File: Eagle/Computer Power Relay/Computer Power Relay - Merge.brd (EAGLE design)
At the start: 133.4 x 78 mm, 141 parts, among them K1 RELAY-3V3DC-110VAC012, K2 RELAY-110VACV3_IN-PLACE, U1 RP2040, U2 AP2112M-3.3TRG1, U3 SWITCH-SLIDE-DPDT, U4 SWITCH-SLIDE-DPDT, U5 SWITCH-SLIDE-DPDT, U6 RP2040, U7 AP2112M-3.3TRG1

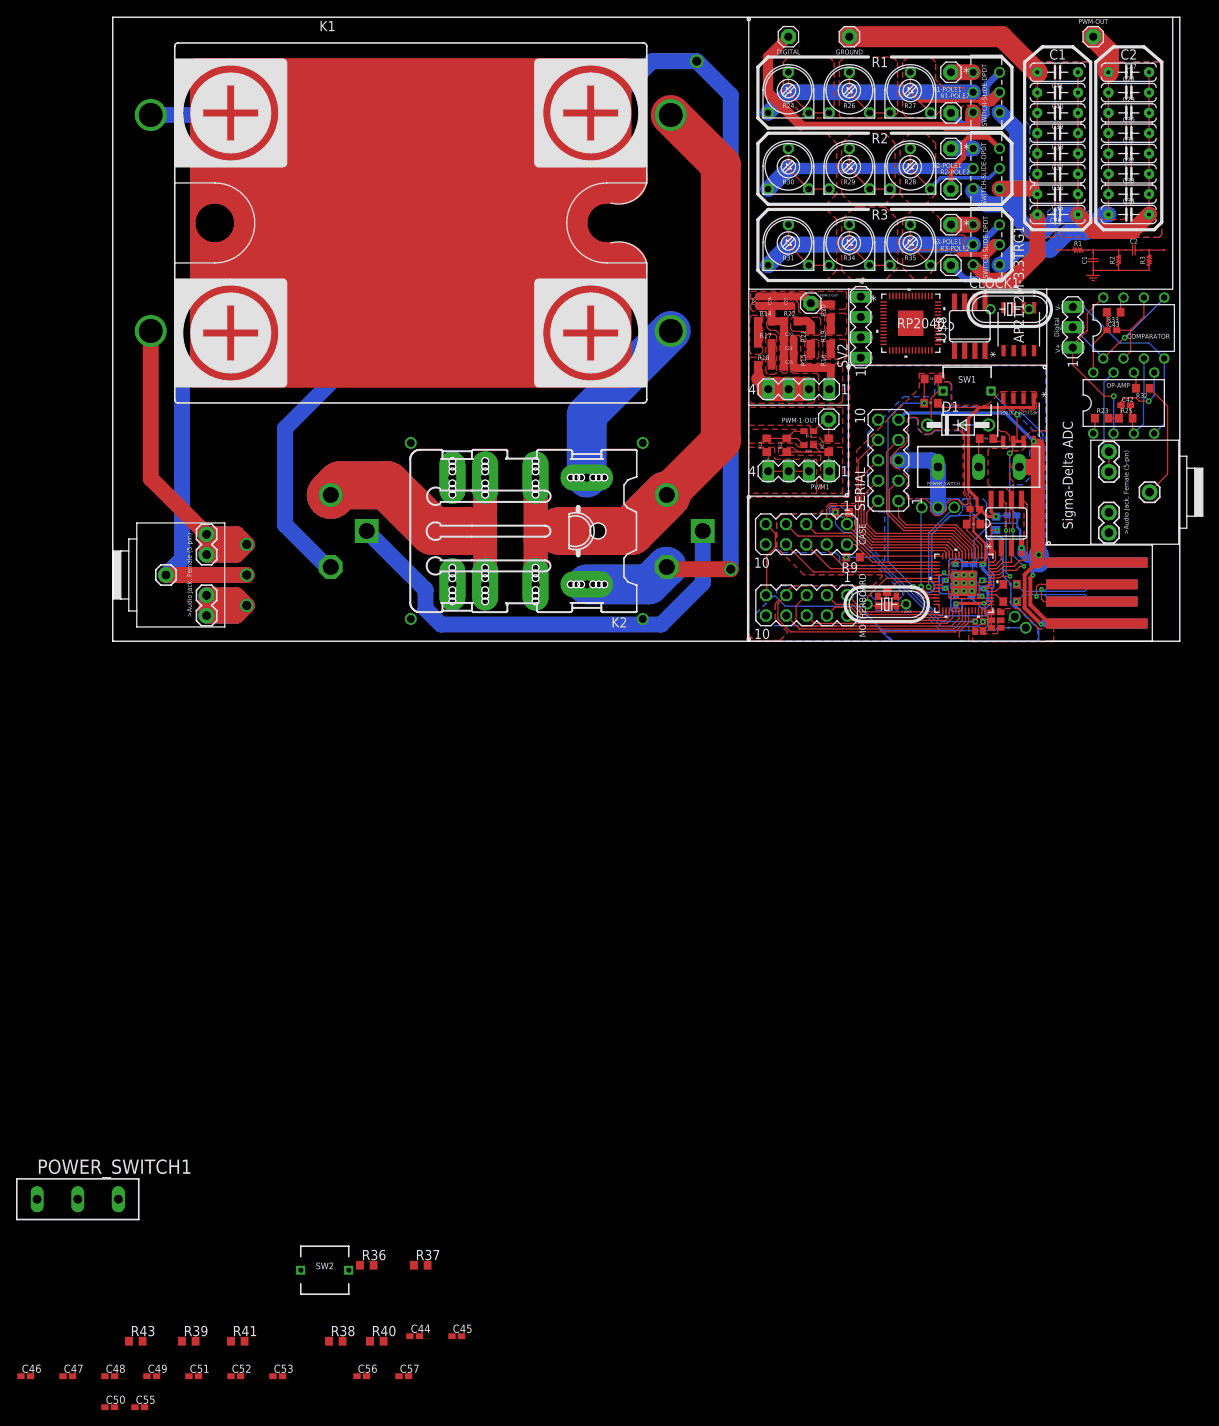
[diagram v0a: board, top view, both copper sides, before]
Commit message: CPR 100% Complete
Damn shipping's expensive.  Better work on the other projects so I can subsidize this.
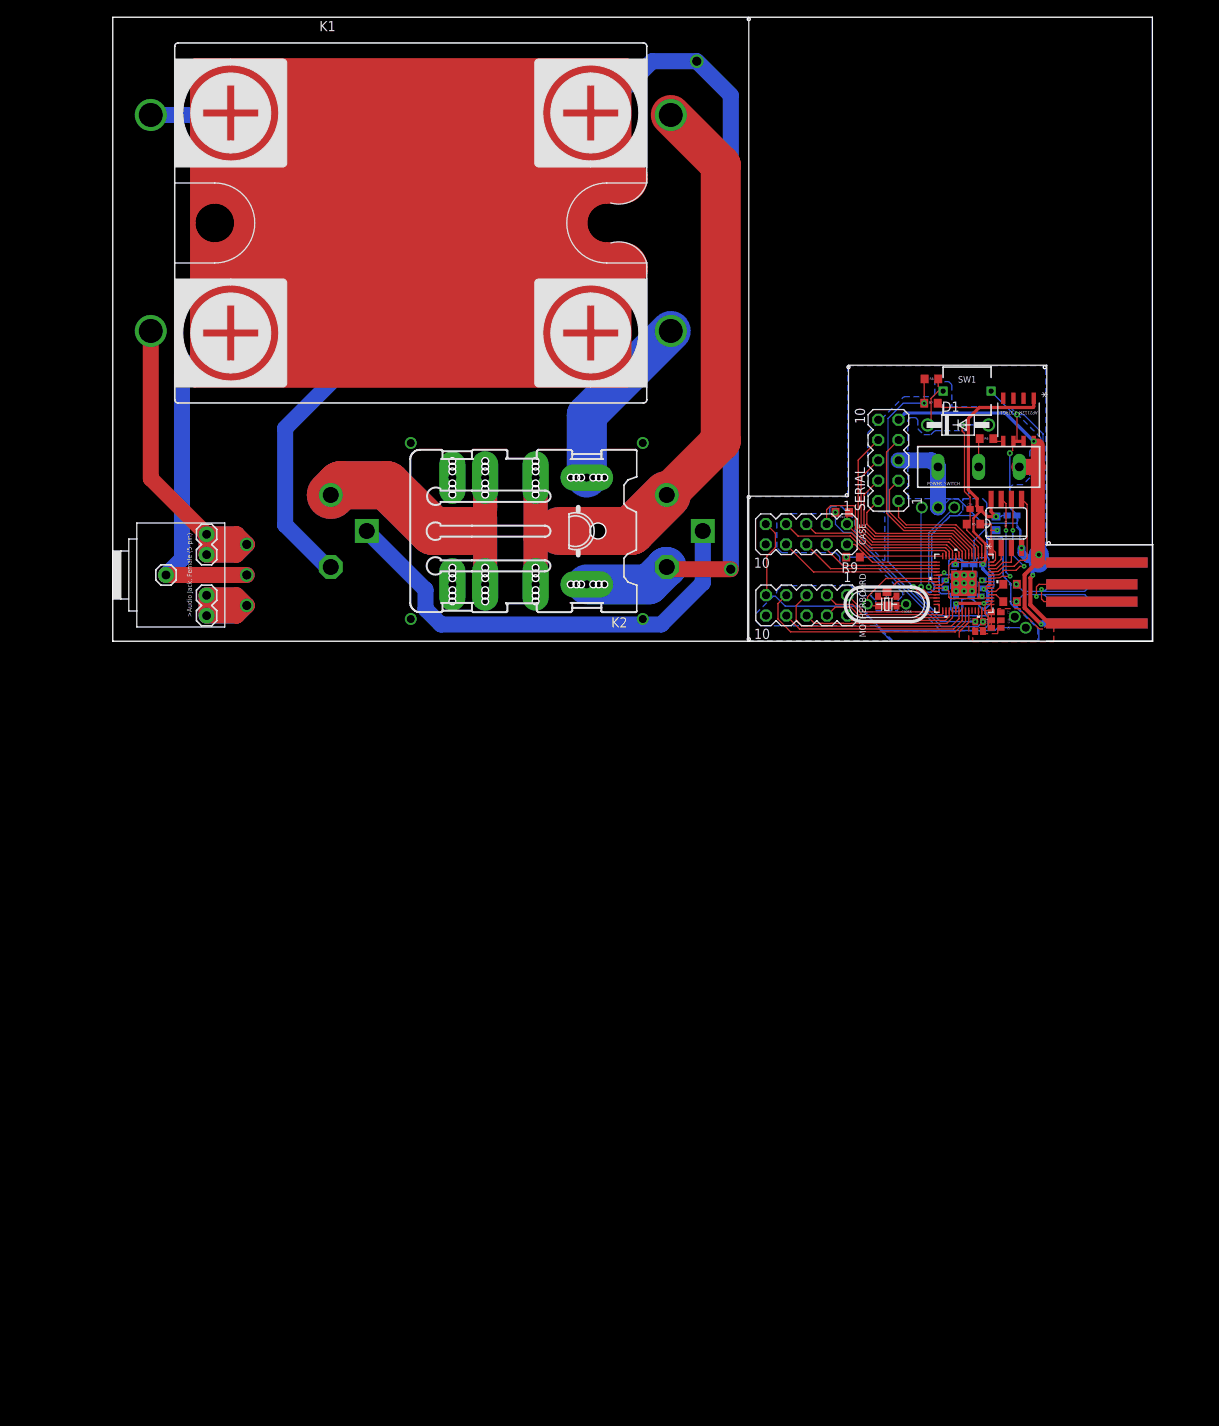
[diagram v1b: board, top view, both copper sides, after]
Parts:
- removed C18, C20, C22, C23, C46, C47, C48, C49, C51, C52, C53, C56, C57: 100nF, adafruit:C0402K
- removed C19, C21, C24, C25: 47uF, adafruit:C0402K
- removed C26, C27, C28, C29, C30, C31, C32, C33, C34, C35, C36, C37, C38, C39, C40, C41: (no value), Inventory:CAPACITOR-CERAMIC
- removed C42, C43: (no value), adafruit:C0402K
- removed C44, C45: ~30pF, adafruit:C0402K
- removed C50, C55: 1uF, adafruit:C0402K
- removed CLOCK1: 12MHz, crystal:HC49/S
- removed COMPARATOR: COMPARATOR_LM393N, Inventory:IC_2*4(8-PIN)
- removed DIGITAL, GROUND, PWM-1-OUT, PWM-2-OUT, PWM-OUT, R1-POLE1, R1-POLE2, R2-POLE1, R2-POLE2, R3-POLE1, R3-POLE2: (no value), adafruit:1X01
- removed OP-AMP: OP-AMP_TDA2822N, Inventory:IC_2*4(8-PIN)
- removed POWER_SWITCH1: SWITCH-SLIDE-2P2T, Inventory:SWITCH-SLIDE-2P2T
- removed PWM1, PWM2, SV2: (no value), con-lstb:MA04-1
- removed R11, R14, R17, R18: 220 Ω, rcl:R0603
- removed R12, R15, R21, R22: 100 Ω, rcl:R0603
- removed R13, R16, R19, R20: 1.8K Ω, rcl:R0603
- removed R23, R25, R32, R33: (no value), rcl:R0603
- removed R24, R30, R31: 1MΩ, Inventory:POTENTIOMETER_NORMAL
- removed R26, R29, R34: 10KΩ, Inventory:POTENTIOMETER_NORMAL
- removed R27, R28, R35: 100Ω, Inventory:POTENTIOMETER_NORMAL
- removed R36, R37: 27.4 Ω, rcl:R0603
- removed R38, R40: 1k Ω, rcl:R0603
- removed R39, R41: 10k Ω, rcl:R0603
- removed R43: 4.7k Ω, rcl:R0603
- removed SV1: (no value), con-lstb:MA03-1
- removed SW2: (no value), KVM Keyboard:PUSHBUTTON_TH
- removed U$6: AUDIO_JACK_FEMALE_5-PIN, Inventory:AUDIO_JACK_FEMALE_5-PIN
- removed U$8: W25Q128JVSIM-ND__QSPI-FLASH, KVM Keyboard:SO08
- removed U3, U4, U5: SWITCH-SLIDE-DPDT, Inventory:SWITCH-SLIDE-DPDT
- removed U6: RP2040, KVM Keyboard:IC57_RP2040
- removed U7: AP2112M-3.3TRG1, KVM Keyboard:AP2112M-3.3TRG1_DIO
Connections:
- removed net 5V_2: POWER_SWITCH1.1, SV2.1, U7.8
- removed net D+_2: R36.2, SV2.3
- removed net D-_2: R37.2, SV2.2
- removed net DIGITAL: COMPARATOR.1, COMPARATOR.5, SV1.2
- removed net GND-3: C18.2, PWM1.1, R12.2, R13.2
- removed net GND-4: C20.2, C22.2, C23.2, PWM2.1, R15.2, R16.2
- removed net GND-5: C26.2, C35.2, C36.2, C37.2, C38.2, C39.2, C40.2, C41.2, GROUND.1, U4.4, U5.3
- removed net GND-6: C43.2, COMPARATOR.2, COMPARATOR.6, R32.1, U$6.3
- removed net GND-7: POWER_SWITCH1.3, SV2.4, U7.6, U7.7
- removed net N$10: C19.1, PWM-1-OUT.1, R13.1
- removed net N$11: C20.1, C21.2, C22.1, C23.1, C24.2, C25.2, R14.1, R22.1
- removed net N$12: C21.1, C24.1, C25.1, PWM-2-OUT.1, R20.1
- removed net N$13: R17.1, R18.1
- removed net N$14: R14.2, R17.2
- removed net N$15: R19.2, R20.2
- removed net N$21: R16.1, R19.1
- removed net N$22: R15.1, R21.1
- removed net N$23: R21.2, R22.2
- removed net N$24: DIGITAL.1, U3.3
- removed net N$25: R24.2, R24.3, R26.1
- removed net N$26: C27.1, C28.1, C29.1, C30.1, C31.1, C32.1, C33.1, C34.1, PWM-OUT.1, U5.4
- removed net N$27: R26.2, R26.3, R27.1
- removed net N$28: R27.2, R27.3, U3.5
- removed net N$29: R24.1, U3.2
- removed net N$30: R1-POLE1.1, U3.1
- removed net N$31: R1-POLE2.1, U3.6
- removed net N$32: R2-POLE2.1, U4.6
- removed net N$33: R2-POLE1.1, U4.1
- removed net N$34: R30.1, U4.2
- removed net N$35: R28.2, R28.3, U4.5
- removed net N$36: R3-POLE2.1, U5.6
- removed net N$37: R3-POLE1.1, U5.1
- removed net N$38: R28.1, R29.2, R29.3
- removed net N$39: R29.1, R30.2, R30.3
- removed net N$40: R31.1, U5.2
- removed net N$41: R34.2, R34.3, R35.1
- removed net N$42: R31.2, R31.3, R34.1
- removed net N$43: R35.2, R35.3, U5.5
- removed net N$44: C26.1, C27.2, C28.2, C29.2, C30.2, C31.2, C32.2, C33.2, C34.2, C35.1, C36.1, C37.1, C38.1, C39.1, C40.1, C41.1, U3.4, U4.3
- removed net N$45: OP-AMP.7, U$6.4, U$6.5
- removed net N$46: R36.1, U6.47
- removed net N$47: OP-AMP.6, R32.2
- removed net N$51: C43.1, OP-AMP.8, R33.2
- removed net N$52: OP-AMP.1, R23.1
- removed net N$53: C42.1, OP-AMP.5, R23.2, R25.1
- removed net N$54: C42.2, COMPARATOR.3, OP-AMP.3, R25.2
- removed net N$55: R37.1, U6.46
- removed net N$56: COMPARATOR.7, R33.1
- removed net N$57: C45.2, CLOCK1.2, R38.1
- removed net N$58: R38.2, U6.21
- removed net N$59: C44.2, CLOCK1.1, U6.20
- removed net N$6: PWM1.2, PWM1.3, PWM1.4, R11.2
- removed net N$60: U$8.3, U6.54
- removed net N$61: U$8.2, U6.55
- removed net N$62: U$8.5, U6.53
- removed net N$63: U$8.6, U6.52
- removed net N$64: U$8.7, U6.51
- removed net N$7: C18.1, C19.2, R11.1, R12.1
- removed net N$8: PWM2.2, PWM2.3, PWM2.4, R18.2
- removed net SD-V+: COMPARATOR.8, OP-AMP.2, SV1.1
- removed net SD-V-: COMPARATOR.4, OP-AMP.4, SV1.3
- net 1V1: no longer C55.2, C56.2, C57.2, U6.23, U6.45, U6.50
- net 3V3: no longer C46.2, C47.2, C48.2, C49.2, C50.2, C51.2, C52.2, C53.2, R39.2, U$8.8, U6.1, U6.10, U6.22, U6.33, U6.42, U6.43, U6.44, U6.48, U6.49, U7.1
- net BOOTSEL: no longer R40.2
- net BUTTON: no longer R43.1, SW2.P$1
- net EN: no longer R41.2, U7.5
- net GND: no longer C44.1, C45.1, C46.1, C47.1, C48.1, C49.1, C50.1, C51.1, C52.1, C53.1, C55.1, C56.1, C57.1, SW2.P$2, U$8.4, U6.19, U6.57
- net QSPI_SS_N: no longer R39.1, R40.1, U$8.1, U6.56
- net RUN: no longer R43.2, U6.26
- net SWITCH: no longer POWER_SWITCH1.2, R41.1
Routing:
- net N$44: track 76.3 -> 0.00 mm
- net GND-5: track 63.4 -> 0.00 mm
- net N$48: track 43.6 -> 0.00 mm
- net N$26: track 39.2 -> 0.00 mm
- net N$24: track 36.8 -> 0.00 mm
- net N$40: track 26.7 -> 0.00 mm
- net N$34: track 26.7 -> 0.00 mm
- net N$29: track 26.7 -> 0.00 mm
- net GND-6: track 25.3 -> 0.00 mm
- net SD-V-: track 24.0 -> 0.00 mm
- net SD-V+: track 21.4 -> 0.00 mm, vias 1 -> 0
- net N$43: track 17.4 -> 0.00 mm
- net N$28: track 16.7 -> 0.00 mm
- net DIGITAL: track 16.3 -> 0.00 mm, vias 1 -> 0
- net N$35: track 15.9 -> 0.00 mm
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- removed copper zone on layer 1, net GND-3
- removed copper zone on layer 1, net GND-4
- removed copper zone on layer 1, net GND-5
- removed copper zone on layer 16, net GND-5
- removed copper zone on layer 1, net N$10
- removed copper zone on layer 1, net N$11
- removed copper zone on layer 1, net N$12
- removed copper zone on layer 1, net N$13
- removed copper zone on layer 1, net N$14
- removed copper zone on layer 1, net N$15
- removed copper zone on layer 1, net N$21
- removed copper zone on layer 1, net N$22
- removed copper zone on layer 1, net N$23
- removed copper zone on layer 1, net N$24
- removed copper zone on layer 1, net N$25
- removed copper zone on layer 1, net N$26
- removed copper zone on layer 16, net N$26
- removed copper zone on layer 1, net N$27
- removed copper zone on layer 1, net N$28
- removed copper zone on layer 1, net N$35
- removed copper zone on layer 1, net N$38
- removed copper zone on layer 1, net N$39
- removed copper zone on layer 1, net N$41
- removed copper zone on layer 1, net N$42
- removed copper zone on layer 1, net N$43
- removed copper zone on layer 1, net N$44
- removed copper zone on layer 16, net N$44
- removed copper zone on layer 1, net N$6
- removed copper zone on layer 1, net N$7
- removed copper zone on layer 1, net N$8
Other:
- board size 133.4 x 78 mm -> 129.9 x 78 mm
- board text removed: "C1"
- board text removed: "C2"
- board text removed: "Digital"
- board text removed: "R1"
- board text removed: "R2"
- board text removed: "R3"
- board text removed: "RPi Pico recommended values PWM"
- board text removed: "Sigma-Delta ADC"
- board text removed: "V+"
- board text removed: "V-"
